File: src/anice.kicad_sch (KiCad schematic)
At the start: 6 parts, among them J1 Conn_02x20_Counter_Clockwise, U1 ECP5U_12_CABGA256

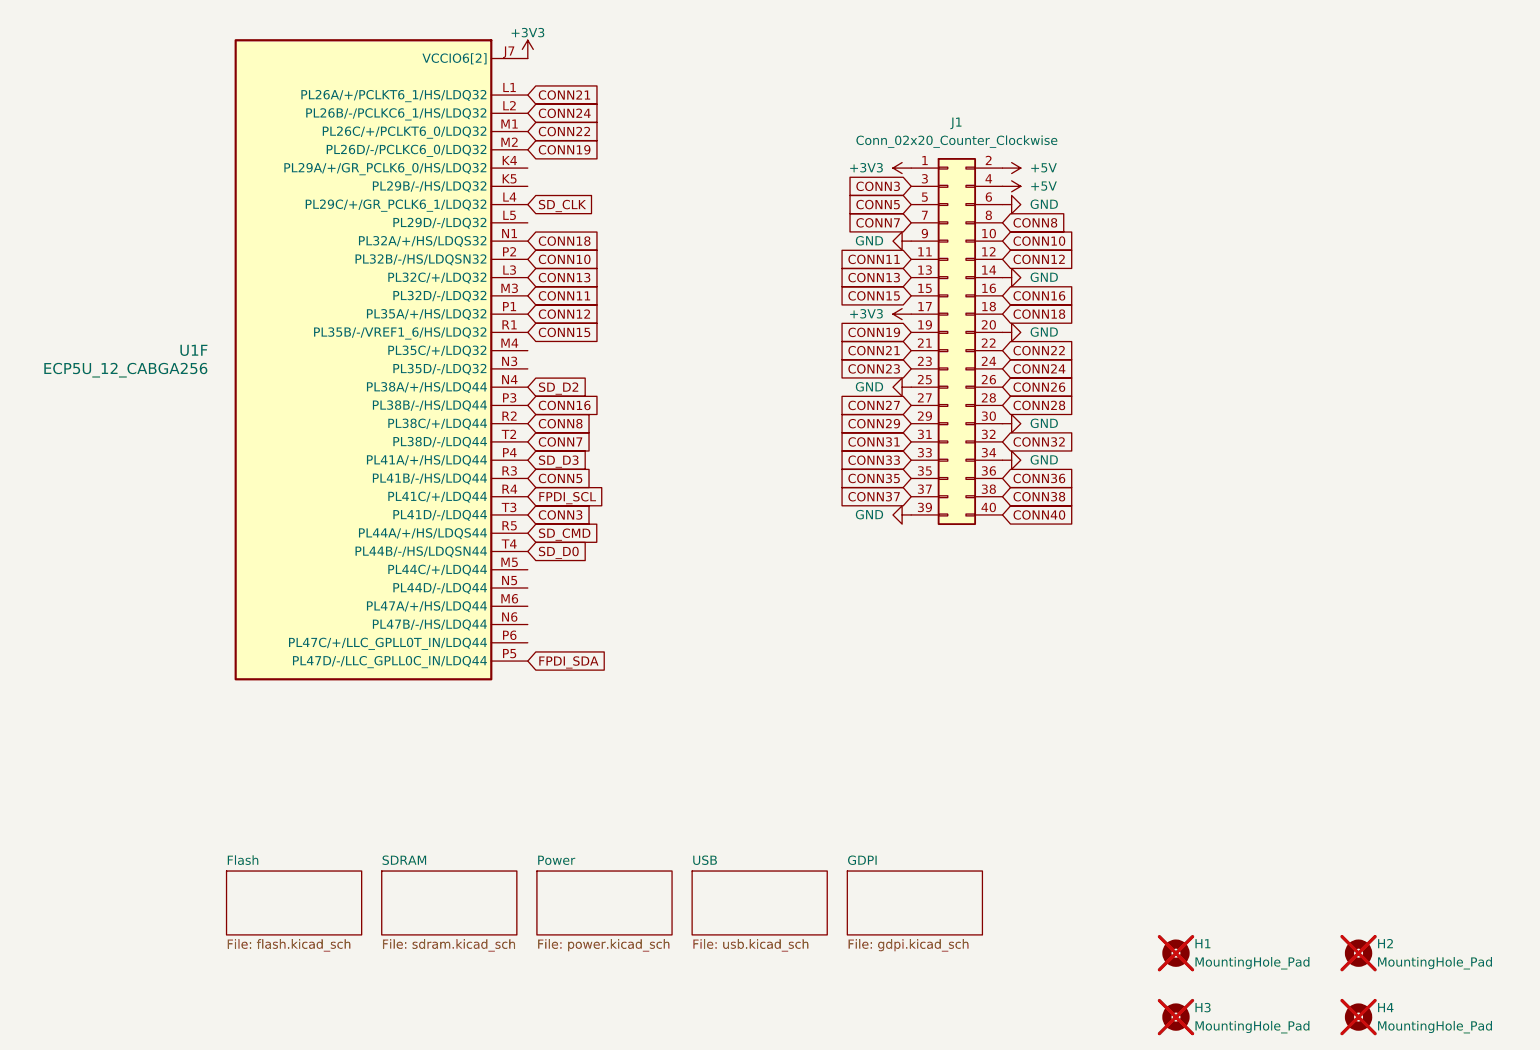
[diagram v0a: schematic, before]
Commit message: Structure project
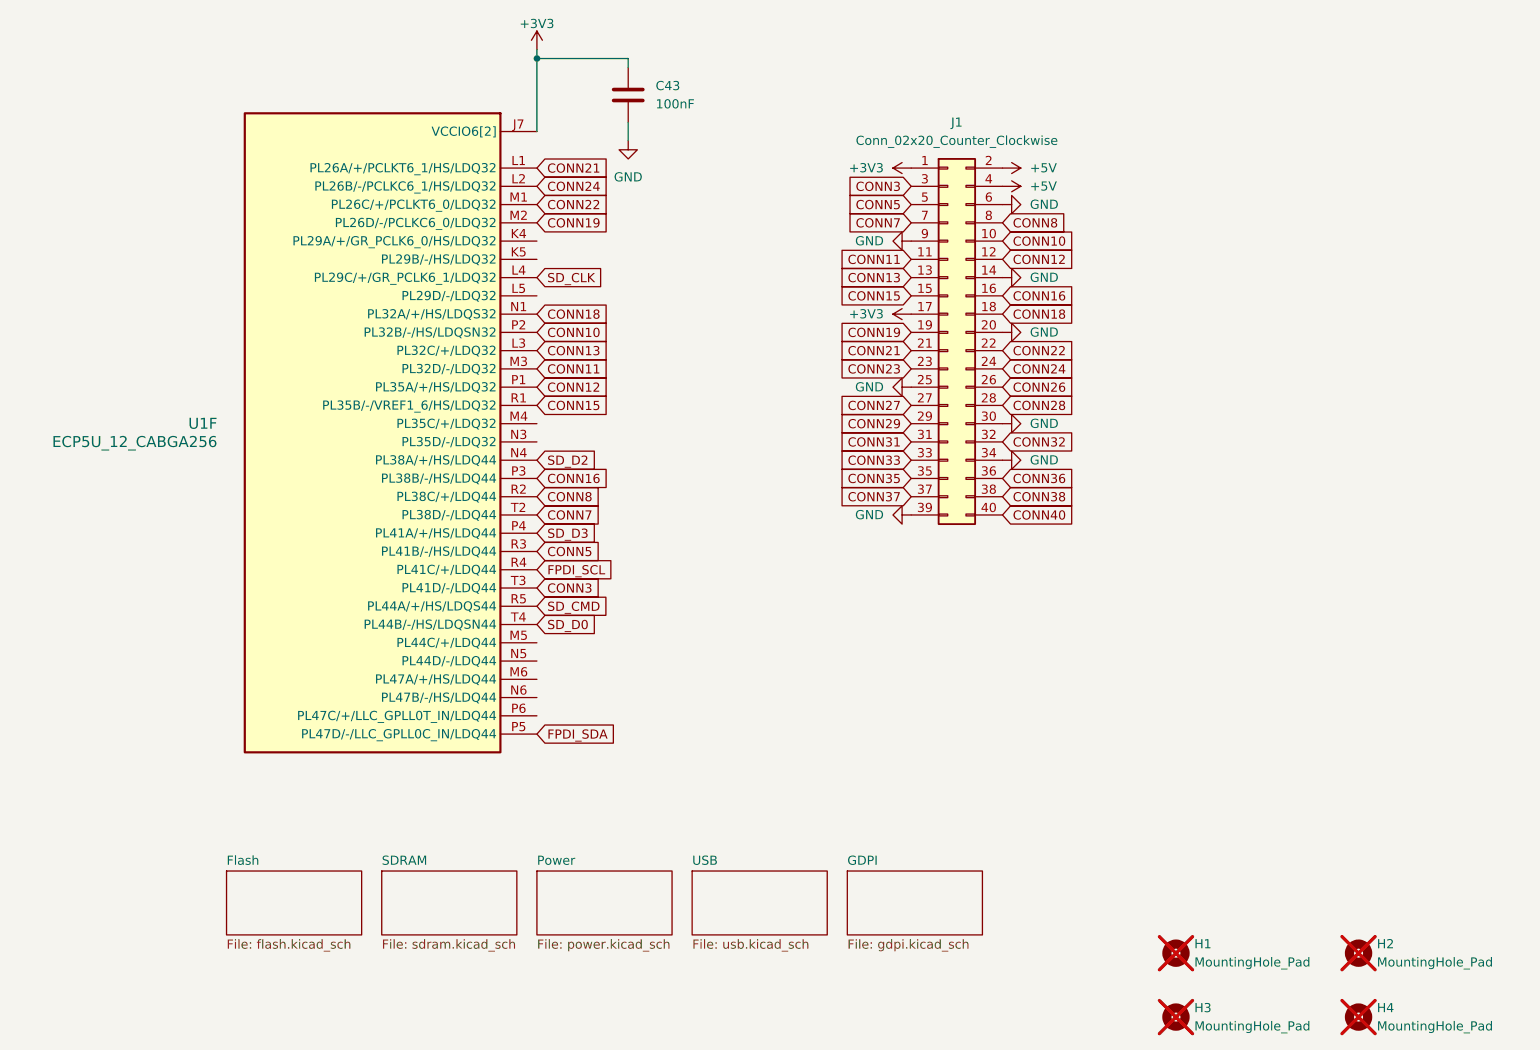
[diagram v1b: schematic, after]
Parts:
- added C43: 100nF, Capacitor_SMD:C_0402_1005Metric, symbol Device:C
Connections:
- net +3V3: now also C43.1
- net GND: now also C43.2
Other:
- moved on the sheet: U1F
